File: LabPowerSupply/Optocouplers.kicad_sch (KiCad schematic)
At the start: 3 parts

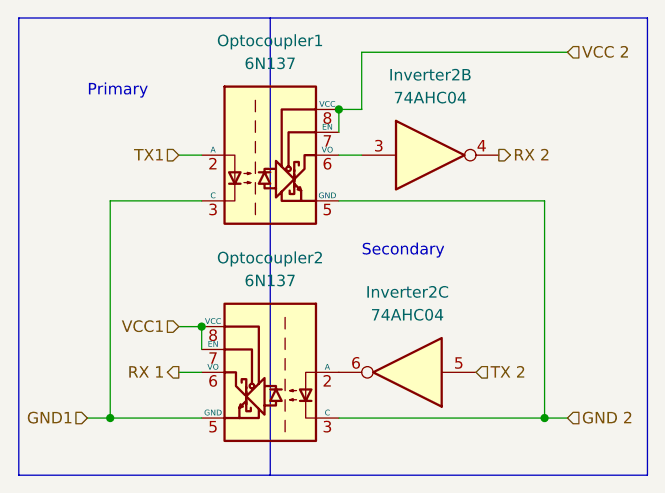
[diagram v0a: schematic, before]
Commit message: Resistor footprints changed to 0603
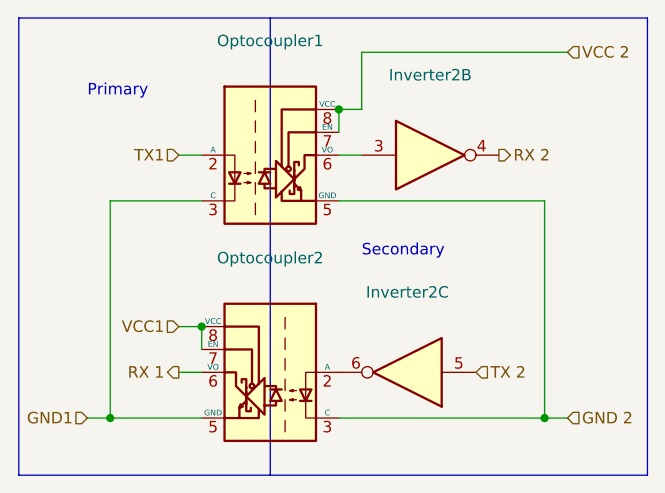
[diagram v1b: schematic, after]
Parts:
- Inverter2: value 74AHC04 -> (none); footprint Package_DIP:DIP-14_W7.62mm -> (none)
- Optocoupler1, Optocoupler2: value 6N137 -> (none); footprint Package_DIP:DIP-8_W7.62mm -> (none)
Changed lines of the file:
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@@
     (in_bom yes) (on_board yes) (fields_autoplaced)
     (property "Reference" "Inverter2" (id 0) (at 142.24 73.66 0))
-    (property "Value" "74AHC04" (id 1) (at 142.24 76.2 0))
-    (property "Footprint" "Package_DIP:DIP-14_W7.62mm" (id 2) (at 142.24 82.55 0)
+    (property "Value" "" (id 1) (at 142.24 76.2 0))
+    (property "Footprint" "" (id 2) (at 142.24 82.55 0)
       (effects (font (size 1.27 1.27)) hide)
     )
@@
     (in_bom yes) (on_board yes) (fields_autoplaced)
     (property "Reference" "Inverter2" (id 0) (at 139.7 97.79 0))
-    (property "Value" "74AHC04" (id 1) (at 139.7 100.33 0))
-    (property "Footprint" "Package_DIP:DIP-14_W7.62mm" (id 2) (at 139.7 106.68 0)
+    (property "Value" "" (id 1) (at 139.7 100.33 0))
+    (property "Footprint" "" (id 2) (at 139.7 106.68 0)
       (effects (font (size 1.27 1.27)) hide)
     )
@@
     (in_bom yes) (on_board yes) (fields_autoplaced)
     (property "Reference" "Optocoupler2" (id 0) (at 124.46 93.98 0))
-    (property "Value" "6N137" (id 1) (at 124.46 96.52 0))
-    (property "Footprint" "Package_DIP:DIP-8_W7.62mm" (id 2) (at 124.46 119.38 0)
+    (property "Value" "" (id 1) (at 124.46 96.52 0))
+    (property "Footprint" "" (id 2) (at 124.46 119.38 0)
       (effects (font (size 1.27 1.27)) hide)
     )
@@
     (in_bom yes) (on_board yes) (fields_autoplaced)
     (property "Reference" "Optocoupler1" (id 0) (at 124.46 69.85 0))
-    (property "Value" "6N137" (id 1) (at 124.46 72.39 0))
-    (property "Footprint" "Package_DIP:DIP-8_W7.62mm" (id 2) (at 124.46 95.25 0)
+    (property "Value" "" (id 1) (at 124.46 72.39 0))
+    (property "Footprint" "" (id 2) (at 124.46 95.25 0)
       (effects (font (size 1.27 1.27)) hide)
     )

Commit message: Added mcu capacitors, split 5v inductors
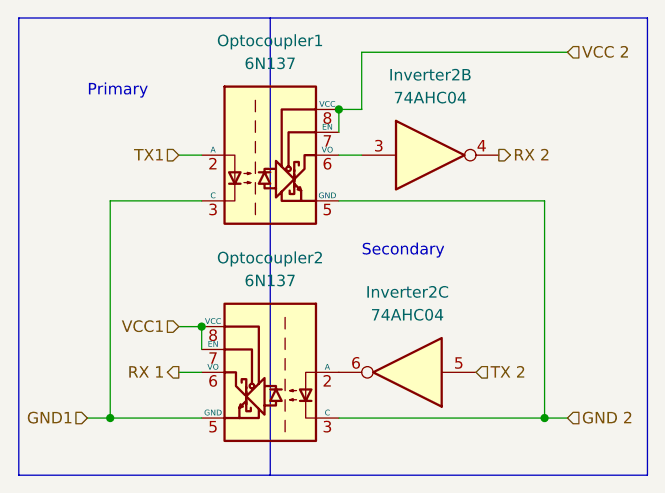
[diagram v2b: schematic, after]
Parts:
- Inverter2: value (none) -> 74AHC04; footprint (none) -> Package_DIP:DIP-14_W7.62mm
- Optocoupler1, Optocoupler2: value (none) -> 6N137; footprint (none) -> Package_DIP:DIP-8_W7.62mm
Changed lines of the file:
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@@
     (in_bom yes) (on_board yes) (fields_autoplaced)
     (property "Reference" "Inverter2" (id 0) (at 142.24 73.66 0))
-    (property "Value" "" (id 1) (at 142.24 76.2 0))
-    (property "Footprint" "" (id 2) (at 142.24 82.55 0)
+    (property "Value" "74AHC04" (id 1) (at 142.24 76.2 0))
+    (property "Footprint" "Package_DIP:DIP-14_W7.62mm" (id 2) (at 142.24 82.55 0)
       (effects (font (size 1.27 1.27)) hide)
     )
@@
     (in_bom yes) (on_board yes) (fields_autoplaced)
     (property "Reference" "Inverter2" (id 0) (at 139.7 97.79 0))
-    (property "Value" "" (id 1) (at 139.7 100.33 0))
-    (property "Footprint" "" (id 2) (at 139.7 106.68 0)
+    (property "Value" "74AHC04" (id 1) (at 139.7 100.33 0))
+    (property "Footprint" "Package_DIP:DIP-14_W7.62mm" (id 2) (at 139.7 106.68 0)
       (effects (font (size 1.27 1.27)) hide)
     )
@@
     (in_bom yes) (on_board yes) (fields_autoplaced)
     (property "Reference" "Optocoupler2" (id 0) (at 124.46 93.98 0))
-    (property "Value" "" (id 1) (at 124.46 96.52 0))
-    (property "Footprint" "" (id 2) (at 124.46 119.38 0)
+    (property "Value" "6N137" (id 1) (at 124.46 96.52 0))
+    (property "Footprint" "Package_DIP:DIP-8_W7.62mm" (id 2) (at 124.46 119.38 0)
       (effects (font (size 1.27 1.27)) hide)
     )
@@
     (in_bom yes) (on_board yes) (fields_autoplaced)
     (property "Reference" "Optocoupler1" (id 0) (at 124.46 69.85 0))
-    (property "Value" "" (id 1) (at 124.46 72.39 0))
-    (property "Footprint" "" (id 2) (at 124.46 95.25 0)
+    (property "Value" "6N137" (id 1) (at 124.46 72.39 0))
+    (property "Footprint" "Package_DIP:DIP-8_W7.62mm" (id 2) (at 124.46 95.25 0)
       (effects (font (size 1.27 1.27)) hide)
     )
